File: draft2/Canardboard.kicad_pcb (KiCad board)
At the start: 4 copper layers, 63.6 x 50.8 mm, 111 parts, among them IC1 SIC437DED-T1-GE3, J1 RBUS, J2 USB_C_Receptacle_USB2.0, J3 Micro_SD_Card_Det, J4 Conn_01x02_Male, J5 Conn_01x03_Male, J6 Conn_01x03_Male, J7 Conn_01x03_Male, Q1 SI4143DY-T1-GE3, Q2 SI4143DY-T1-GE3, U1 ESP32-S3, U10 LTC4412xS6, U2 SN65HVD230, U3 LM66200DRLR, U5 MAX77827AEFD+T, U6 SC4215, U7 ICM-20608-G, U8 MMC5983MA, U9 LTC4412xS6, Y1 40MHz±10ppm

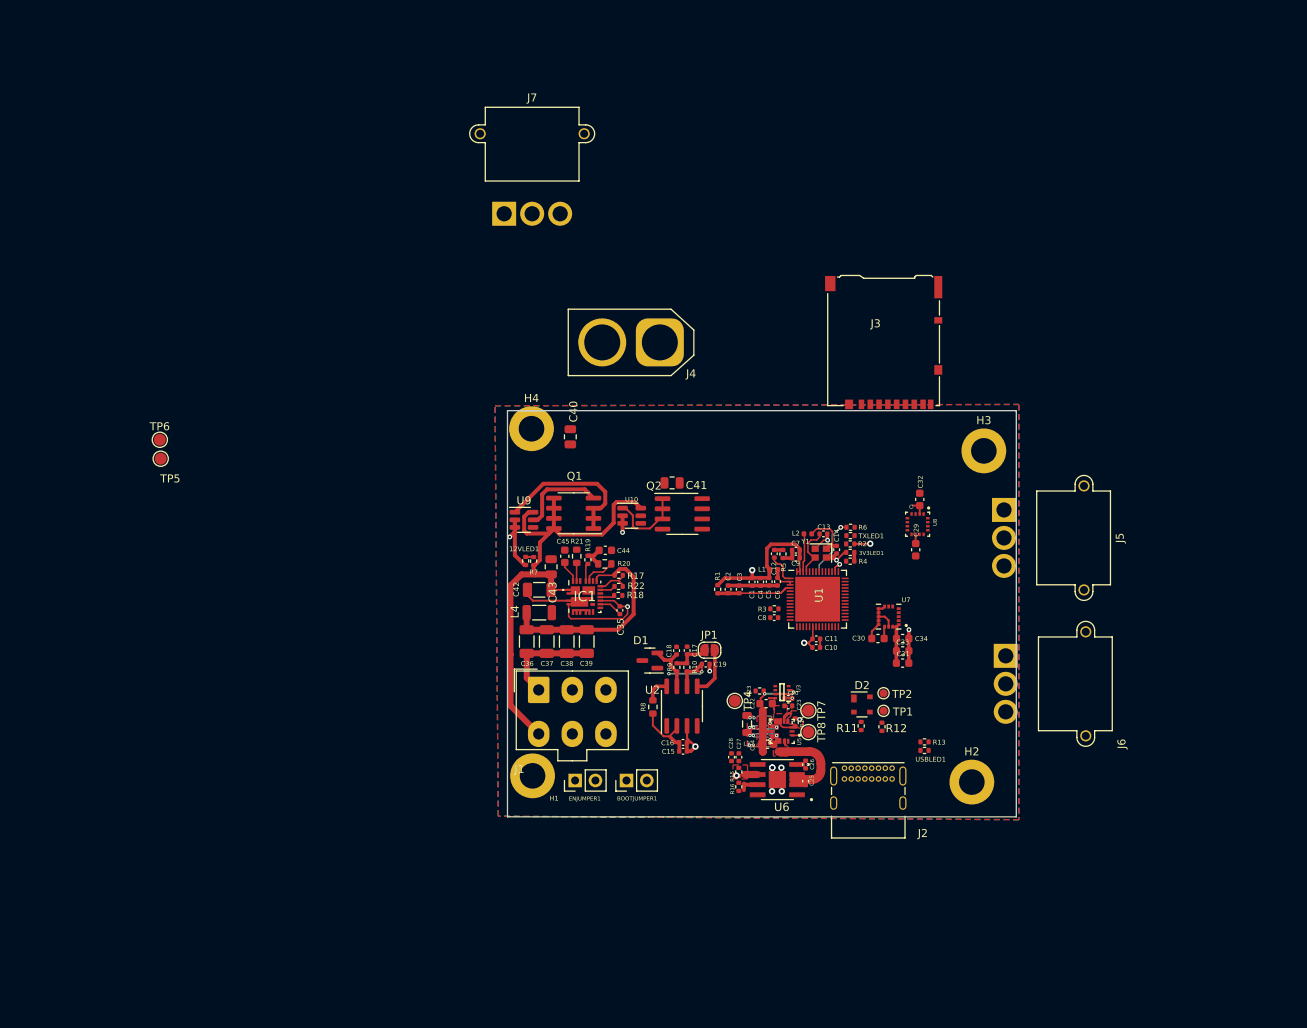
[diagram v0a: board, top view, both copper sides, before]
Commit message: 04/02/2023
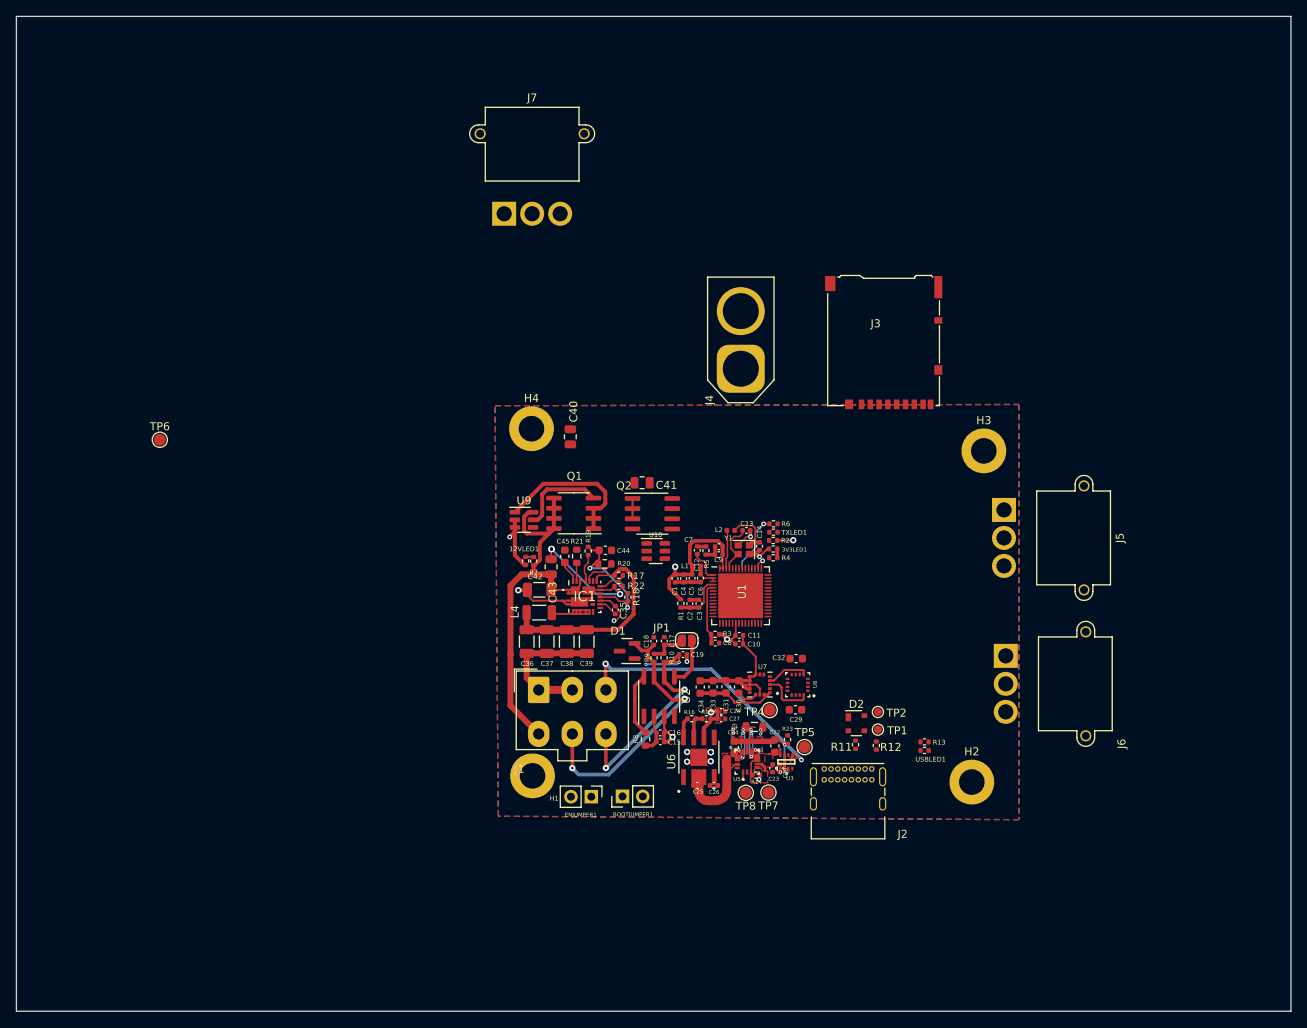
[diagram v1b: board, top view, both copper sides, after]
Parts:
- moved TP5 88.2 mm to (134.7, 116.8)
- moved C34 26.0 mm to (121.7, 109.3), turned to 90 degrees
- moved C32 25.2 mm to (133.6, 105.8), turned to 180 degrees
- moved U8 25.1 mm to (133.8, 109.0), turned to 180 degrees
- moved C29 25.0 mm to (133.6, 112.2), turned to 0 degrees
- moved C33 24.1 mm to (123.2, 109.3), turned to 90 degrees
- moved C31 22.3 mm to (124.9, 109.3), turned to 90 degrees
- moved C30 18.4 mm to (126.5, 109.3), turned to 90 degrees
- moved U7 18.2 mm to (129.1, 109.0)
- moved C25 13.5 mm to (121.3, 121.6), turned to 180 degrees
- moved C26 11.8 mm to (123.4, 121.6), turned to 0 degrees
- moved TP7 11.4 mm to (130.2, 122.5), turned to 180 degrees
- moved TP8 10.9 mm to (127.3, 122.5), turned to 180 degrees
- moved J4 10.6 mm to (126.7, 69.5), turned to 90 degrees
- moved R16 10.4 mm to (120.6, 113.3), turned to 180 degrees
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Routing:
- net RBUS_uC_V: track 0.00 -> 37.1 mm, vias 0 -> 2
- net /CAN+: track 6.70 -> 34.7 mm, vias 0 -> 2
- net /CAN-: track 11.2 -> 33.0 mm, vias 2 -> 4
- net GNDA: track 1.96 -> 16.9 mm, vias 0 -> 3
- net +12V: track 62.8 -> 49.5 mm
- net Net-(C44-Pad1): track 5.21 -> 18.2 mm, vias 0 -> 2
- net /BOOT: track 0.00 -> 7.75 mm
- net Net-(J4-Pad1): track 9.87 -> 2.92 mm
- net /SPI_MOSI: track 0.00 -> 6.48 mm
- net /SPI_MISO: track 0.00 -> 5.32 mm
- net Net-(C31-Pad1): track 5.43 -> 10.4 mm
- net /comps/SW: track 0.00 -> 4.74 mm
- net Net-(R8-Pad1): track 3.24 -> 7.98 mm
- net /CHIP_PU: track 10.3 -> 6.28 mm
- net +3V3: track 38.3 -> 40.2 mm, vias 6 -> 5
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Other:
- board size 63.6 x 50.8 mm -> 159.3 x 124.4 mm
